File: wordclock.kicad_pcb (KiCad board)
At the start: 2 copper layers, 33 x 63.5 mm, 24 parts, among them CON1 AVR-ISP-6, J1 UART, J2 Jack-DC, J3 Screw_Terminal_01x03, SW1 SW_Push, SW2 SW_Push, U1 ATMEGA168PA-PU, U2 DS1307+, Y1 16MHz, Y2 32.7680kHz

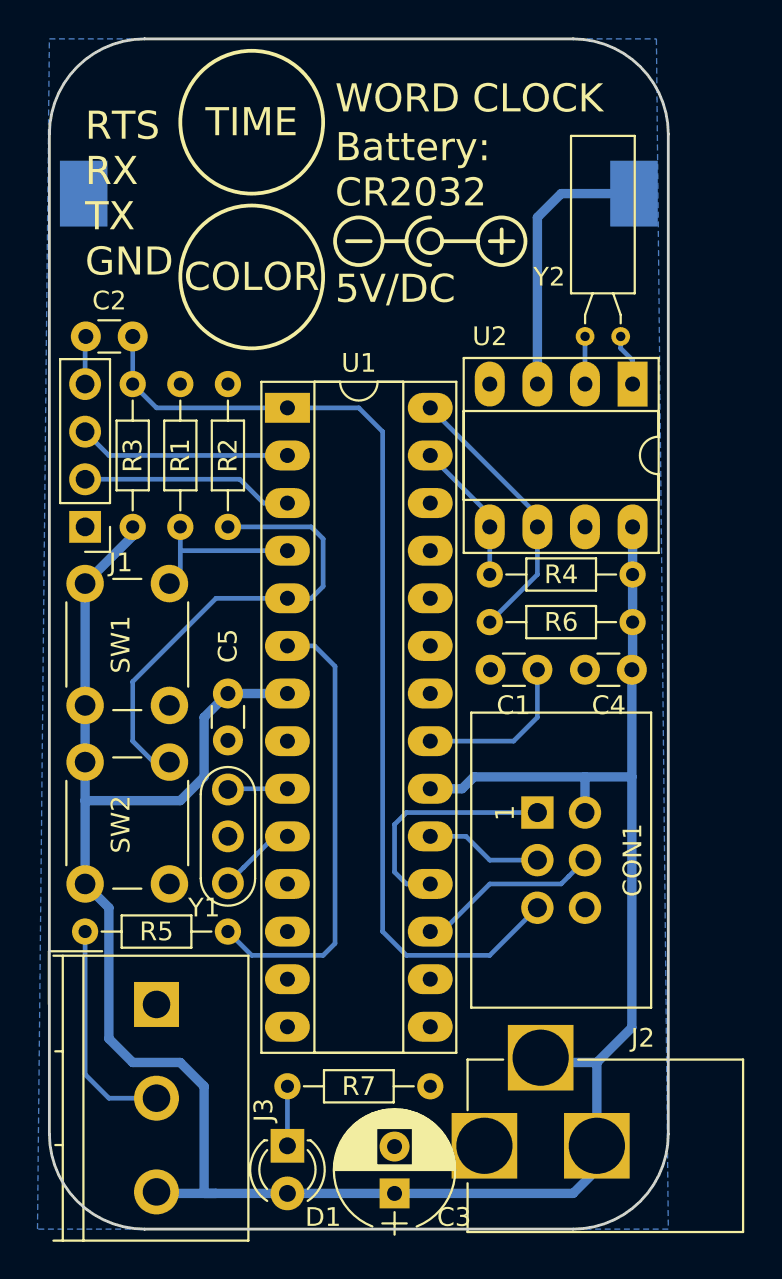
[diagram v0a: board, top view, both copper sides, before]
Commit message: added ignore file
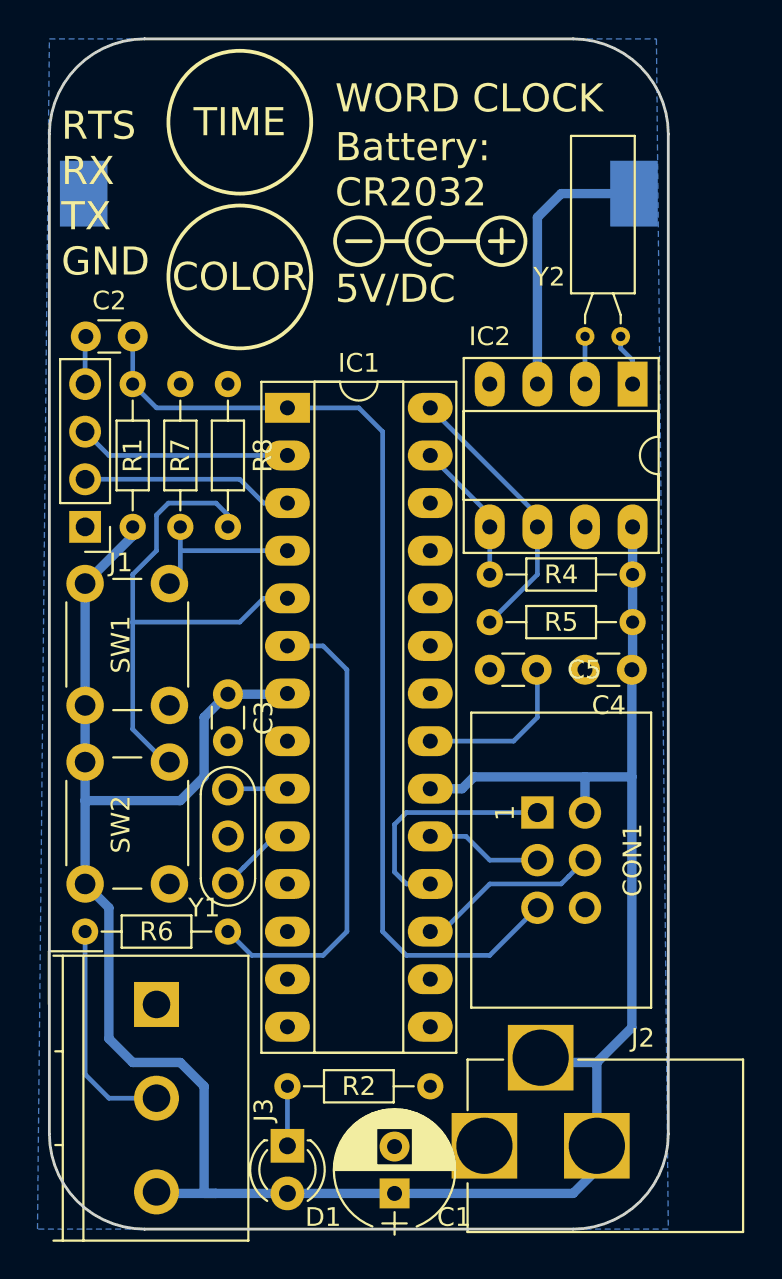
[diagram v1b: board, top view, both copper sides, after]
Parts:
- removed the R7 at (34.3, 168.3)
- removed U1: ATMEGA168PA-PU, Housings_DIP:DIP-28_W7.62mm_Socket_LongPads
- added IC1: ATMEGA168PA-PU, Housings_DIP:DIP-28_W7.62mm_Socket_LongPads, F.Cu at (34.3, 132.1)
- added R8: 10k, Resistors_THT:R_Axial_DIN0204_L3.6mm_D1.6mm_P7.62mm_Horizontal, F.Cu at (31.1, 130.8)
- J1: value UART -> UAR7
- J3: value Screw_Terminal_01x03 -> Neo Pixel
- Y2: footprint Crystals:Crystal_C38-LF_d3.0mm_l8.0mm_Horizontal -> Crystals:Crystal_C18-LF_d3.0mm_l8.0mm_Horizontal
- moved R2 37.6 mm to (34.3, 168.3), turned to 0 degrees
- moved C3 16.6 mm to (31.1, 147.4), turned to 270 degrees
- moved C5 16.5 mm to (47.6, 146.1), turned to 180 degrees
- renumbered C3 to C1, C1 to C3, U2 to IC2, R3 to R1, R6 to R5, R5 to R6, R1 to R7
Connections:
- net /RTS renamed /R7S
- C3 pad 1: Net-(C1-Pad1) -> +5V
- C5 pad 1: +5V -> Net-(C5-Pad1)
- R2 pad 1: GND -> Net-(D1-Pad1)
- R2 pad 2: COLOR -> GND
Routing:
- net Net-(C1-Pad1): track 9.42 -> 0.00 mm
- net Net-(C5-Pad1): track 0.00 -> 8.80 mm
- net COLOR: track 26.0 -> 29.2 mm
- net WS2812: track 24.3 -> 25.1 mm

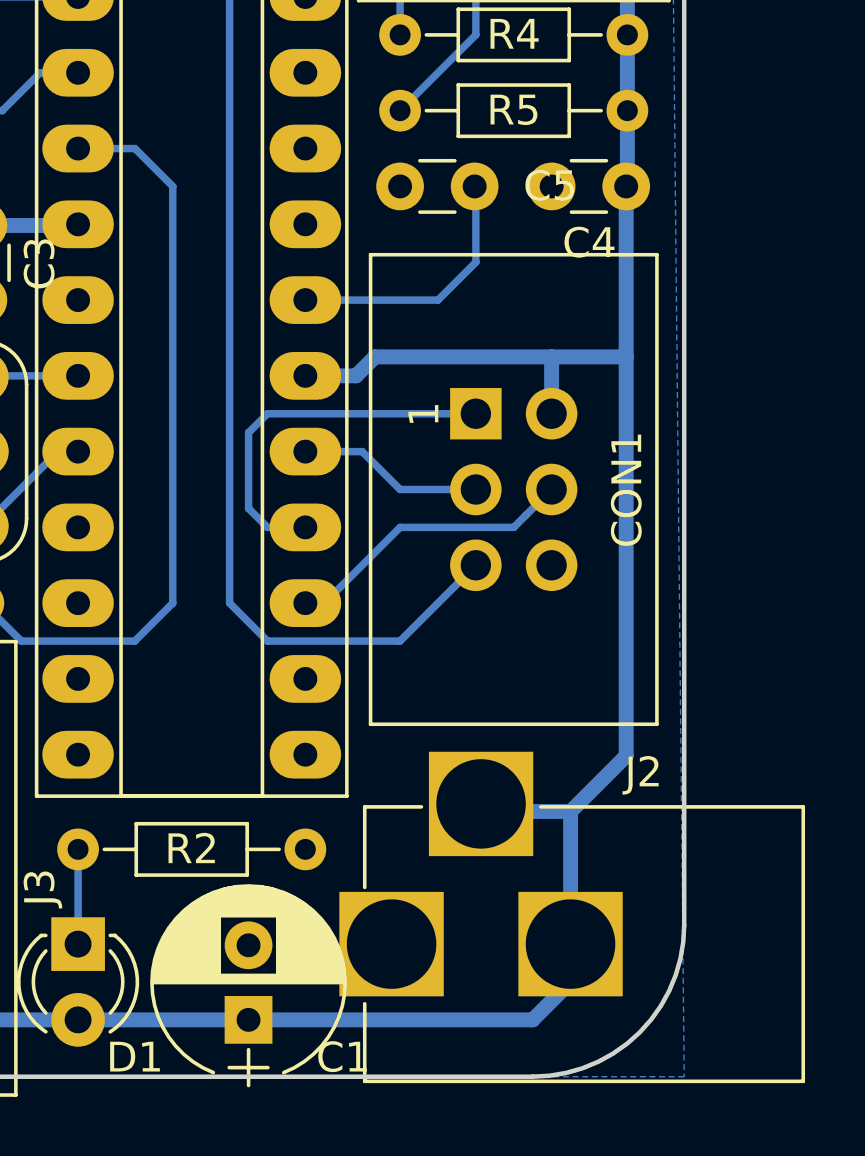
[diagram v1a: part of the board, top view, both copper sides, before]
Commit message: cheanges in wordclock pcb files
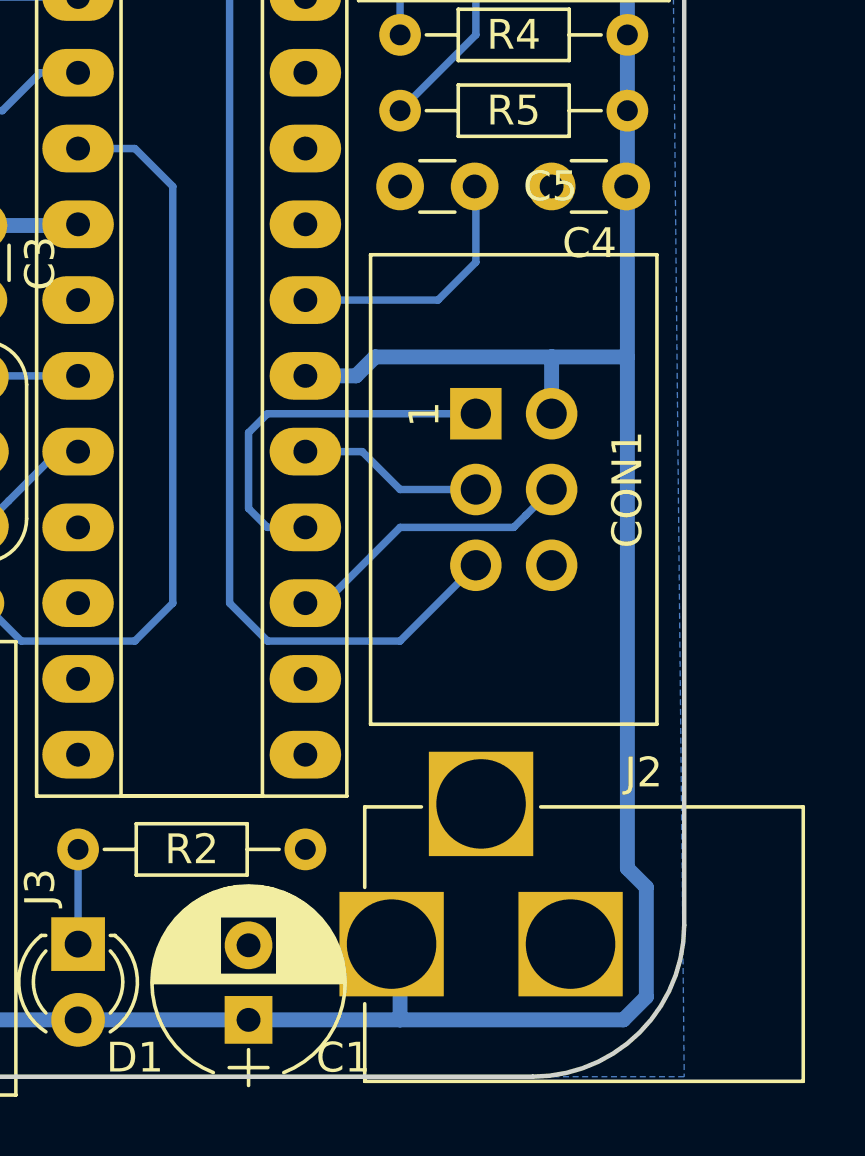
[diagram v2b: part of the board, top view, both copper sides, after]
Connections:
- J2 pad 1: GND -> +5V
- J2 pad 2: +5V -> GND
- J2 pad 3: +5V -> GND
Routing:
- net GND: track 0.00 -> 2.47 mm
- net +5V: track 131.5 -> 133.6 mm
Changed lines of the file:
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@@
   (general
     (links 60)
-    (no_connects 3)
+    (no_connects 2)
     (area 21.514999 112.319999 54.685001 175.970001)
     (thickness 1.6)
     (drawings 25)
-    (tracks 126)
+    (tracks 130)
     (zones 0)
     (modules 24)
@@
     (fp_line (start 0.8 -4.5) (end -13.7 -4.5) (layer F.Fab) (width 0.1))
     (pad 1 thru_hole rect (at 0 0 180) (size 3.5 3.5) (drill 3) (layers *.Cu *.Mask)
-      (net 2 GND))
+      (net 6 +5V))
     (pad 2 thru_hole rect (at -6 0 180) (size 3.5 3.5) (drill 3) (layers *.Cu *.Mask)
-      (net 6 +5V))
+      (net 2 GND))
     (pad 3 thru_hole rect (at -3 4.7 180) (size 3.5 3.5) (drill 3) (layers *.Cu *.Mask)
-      (net 6 +5V))
+      (net 2 GND))
   )
   (module Connectors_Terminal_Blocks:TerminalBlock_Philmore_TB133_03x5mm_Straight (layer F.Cu)
@@
   (segment (start 47.625 121.92) (end 48.895 120.65) (width 0.5) (layer B.Cu) (net 1))
   (segment (start 48.895 120.65) (end 52.78 120.65) (width 0.5) (layer B.Cu) (net 1))
+  (segment (start 50.8 172.72) (end 50.8 171.45) (width 0.5) (layer B.Cu) (net 2))
+  (segment (start 48.895 167.005) (end 48.64 166.75) (width 0.5) (layer B.Cu) (net 2))
+  (segment (start 48.64 166.75) (end 47.8 166.75) (width 0.5) (layer B.Cu) (net 2))
   (segment (start 38.1 132.08) (end 34.29 132.08) (width 0.25) (layer B.Cu) (net 3))
   (segment (start 39.37 133.35) (end 38.1 132.08) (width 0.25) (layer B.Cu) (net 3))
@@
   (segment (start 40.005 156.845) (end 40.64 157.48) (width 0.25) (layer B.Cu) (net 5))
   (segment (start 40.64 157.48) (end 41.91 157.48) (width 0.25) (layer B.Cu) (net 5))
+  (segment (start 45.085 173.99) (end 45.085 171.45) (width 0.5) (layer B.Cu) (net 6))
+  (segment (start 45.085 171.45) (end 44.8 171.45) (width 0.5) (layer B.Cu) (net 6))
+  (segment (start 45.085 173.99) (end 52.570002 173.99) (width 0.5) (layer B.Cu) (net 6))
+  (segment (start 40.005 173.99) (end 45.085 173.99) (width 0.5) (layer B.Cu) (net 6))
+  (segment (start 52.570002 173.99) (end 53.34 173.220002) (width 0.5) (layer B.Cu) (net 6))
+  (segment (start 52.705 168.91) (end 52.705 151.765) (width 0.5) (layer B.Cu) (net 6))
+  (segment (start 53.34 173.220002) (end 53.34 169.545) (width 0.5) (layer B.Cu) (net 6))
+  (segment (start 53.34 169.545) (end 52.705 168.91) (width 0.5) (layer B.Cu) (net 6))
+  (segment (start 52.665 146.05) (end 52.665 146.645) (width 0.5) (layer B.Cu) (net 6))
+  (segment (start 52.665 146.645) (end 52.705 146.685) (width 0.5) (layer B.Cu) (net 6))
+  (segment (start 52.705 146.685) (end 52.705 151.765) (width 0.5) (layer B.Cu) (net 6))
+  (segment (start 50.165 151.765) (end 52.705 151.765) (width 0.5) (layer B.Cu) (net 6))
   (segment (start 23.495 153.035) (end 28.575 153.035) (width 0.5) (layer B.Cu) (net 6))
   (segment (start 29.845 148.59) (end 31.075 147.36) (width 0.5) (layer B.Cu) (net 6))
@@
   (segment (start 24.765 165.735) (end 24.765 158.75) (width 0.5) (layer B.Cu) (net 6))
   (segment (start 24.765 158.75) (end 23.495 157.48) (width 0.5) (layer B.Cu) (net 6))
-  (segment (start 40.005 173.99) (end 49.53 173.99) (width 0.5) (layer B.Cu) (net 6))
-  (segment (start 49.53 173.99) (end 50.8 172.72) (width 0.5) (layer B.Cu) (net 6))
   (segment (start 34.29 173.99) (end 40.005 173.99) (width 0.5) (layer B.Cu) (net 6))
-  (segment (start 50.8 172.72) (end 50.8 171.45) (width 0.5) (layer B.Cu) (net 6))
   (segment (start 30.48 173.99) (end 27.385 173.99) (width 0.5) (layer B.Cu) (net 6))
   (segment (start 34.29 173.99) (end 30.48 173.99) (width 0.5) (layer B.Cu) (net 6))
   (segment (start 27.385 173.99) (end 27.305 173.91) (width 0.5) (layer B.Cu) (net 6))
-  (segment (start 52.665 151.765) (end 52.665 165.14) (width 0.5) (layer B.Cu) (net 6))
-  (segment (start 52.665 165.14) (end 50.8 167.005) (width 0.5) (layer B.Cu) (net 6))
-  (segment (start 50.8 171.45) (end 50.8 167.005) (width 0.5) (layer B.Cu) (net 6))
-  (segment (start 50.8 167.005) (end 48.895 167.005) (width 0.5) (layer B.Cu) (net 6))
-  (segment (start 48.895 167.005) (end 48.64 166.75) (width 0.5) (layer B.Cu) (net 6))
-  (segment (start 48.64 166.75) (end 47.8 166.75) (width 0.5) (layer B.Cu) (net 6))
   (segment (start 23.495 150.98) (end 23.495 153.035) (width 0.5) (layer B.Cu) (net 6))
   (segment (start 23.495 153.035) (end 23.495 157.48) (width 0.5) (layer B.Cu) (net 6))
@@
   (segment (start 26.035 138.43) (end 26.035 138.915) (width 0.5) (layer B.Cu) (net 6))
   (segment (start 26.035 138.915) (end 23.495 141.455) (width 0.5) (layer B.Cu) (net 6))
-  (segment (start 52.665 146.05) (end 52.665 151.765) (width 0.5) (layer B.Cu) (net 6))
-  (segment (start 50.165 151.765) (end 52.665 151.765) (width 0.5) (layer B.Cu) (net 6))
   (segment (start 41.91 152.4) (end 43.61 152.4) (width 0.5) (layer B.Cu) (net 6))
   (segment (start 43.61 152.4) (end 44.245 151.765) (width 0.5) (layer B.Cu) (net 6))
